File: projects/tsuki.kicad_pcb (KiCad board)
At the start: 2 copper layers, 19 parts

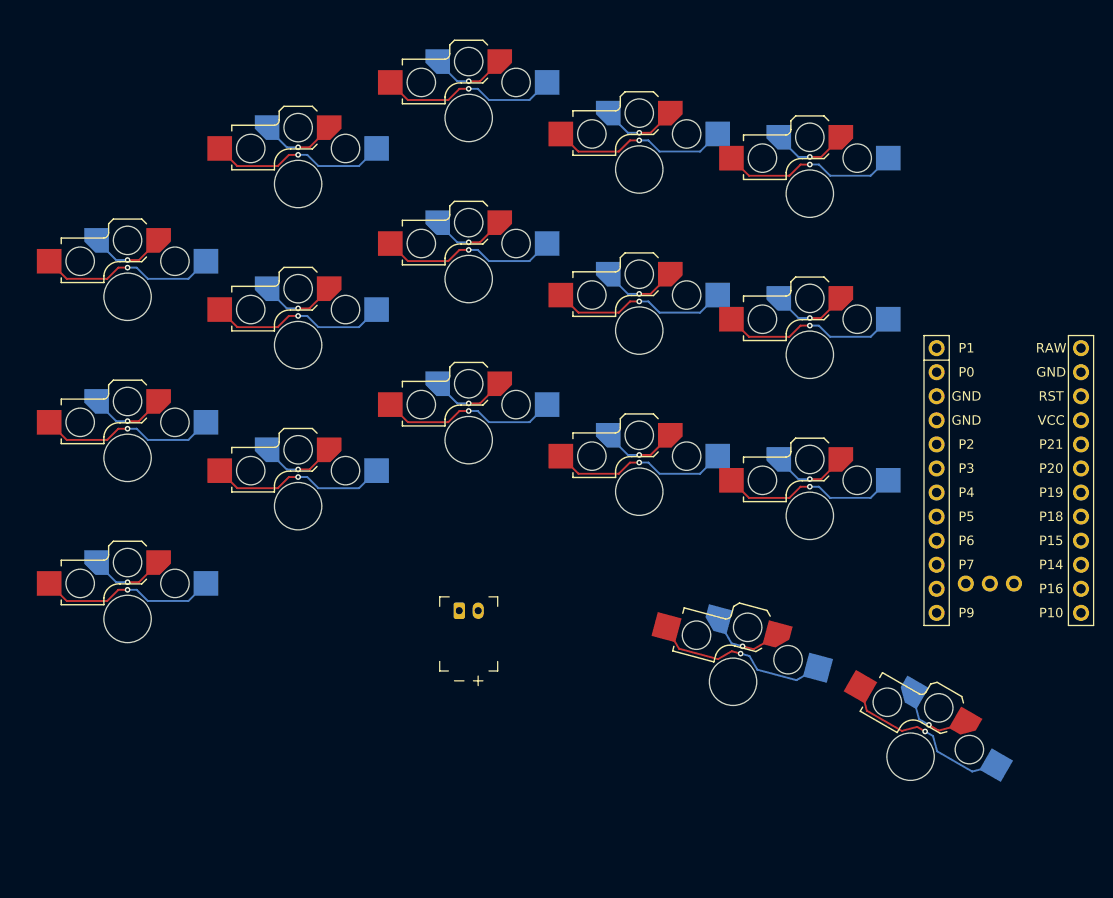
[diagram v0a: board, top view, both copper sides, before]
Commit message: outline in kicad
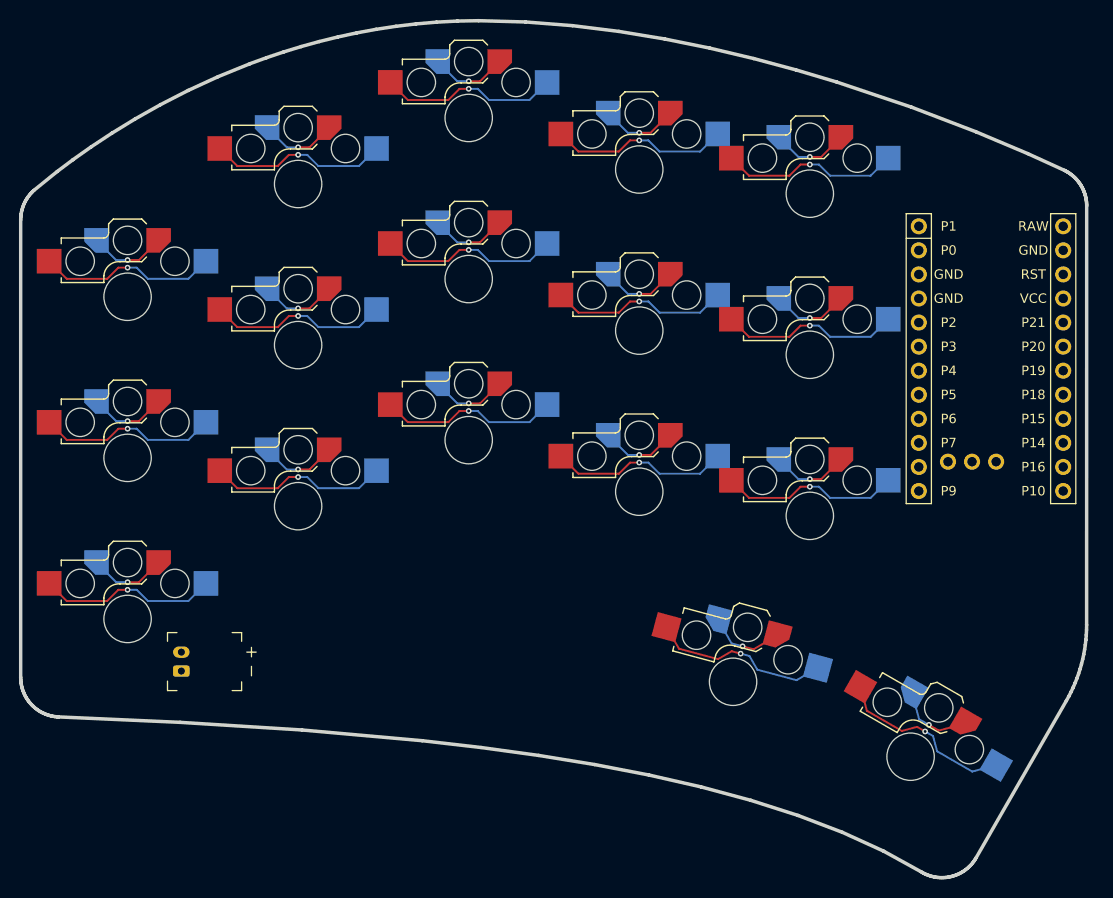
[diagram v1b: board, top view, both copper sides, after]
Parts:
- moved JST1 30.8 mm to (155.7, 154.5), turned to 90 degrees
- moved MCU1 13.0 mm to (241.1, 121.3)
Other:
- board outline added: 112.5 x 90.4 mm
